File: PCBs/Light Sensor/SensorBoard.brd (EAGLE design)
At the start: 69.8 x 56.8 mm, 21 parts, among them J1 AVR_SPI_PRG_6PTH

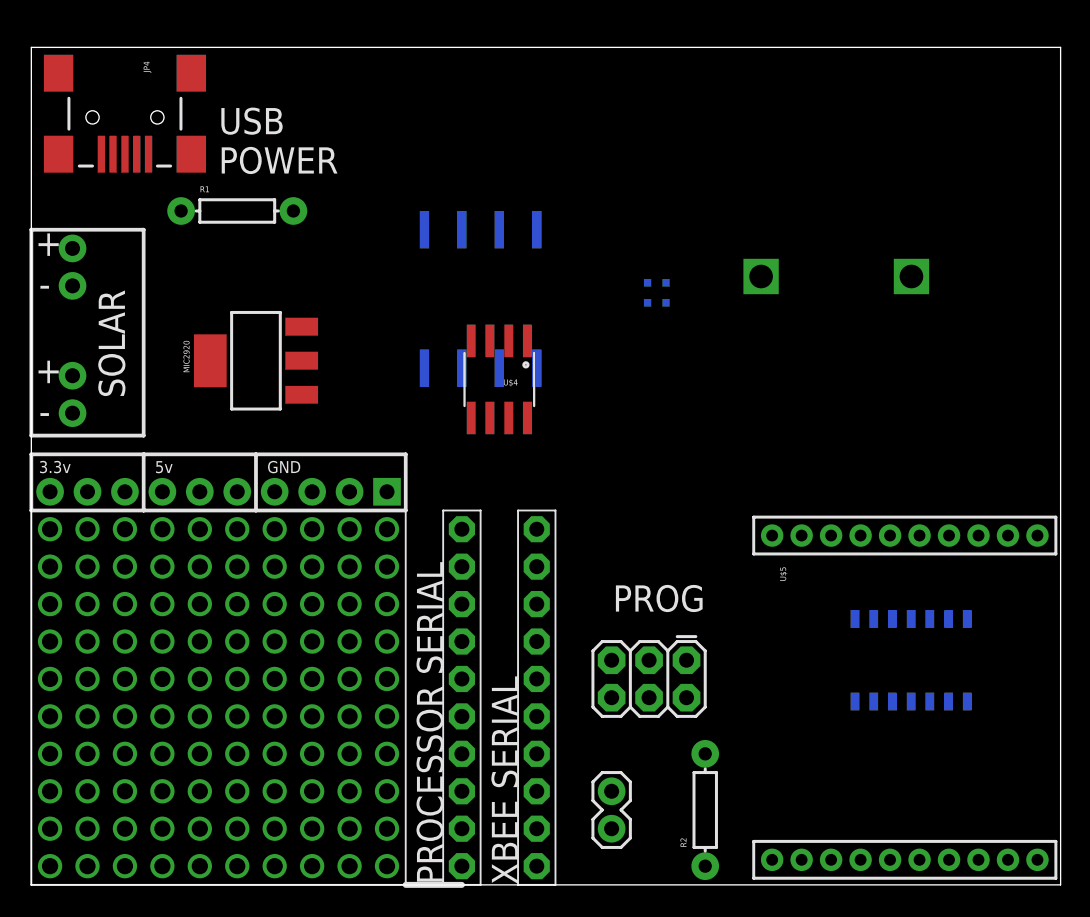
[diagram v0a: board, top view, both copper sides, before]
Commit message: Working layout
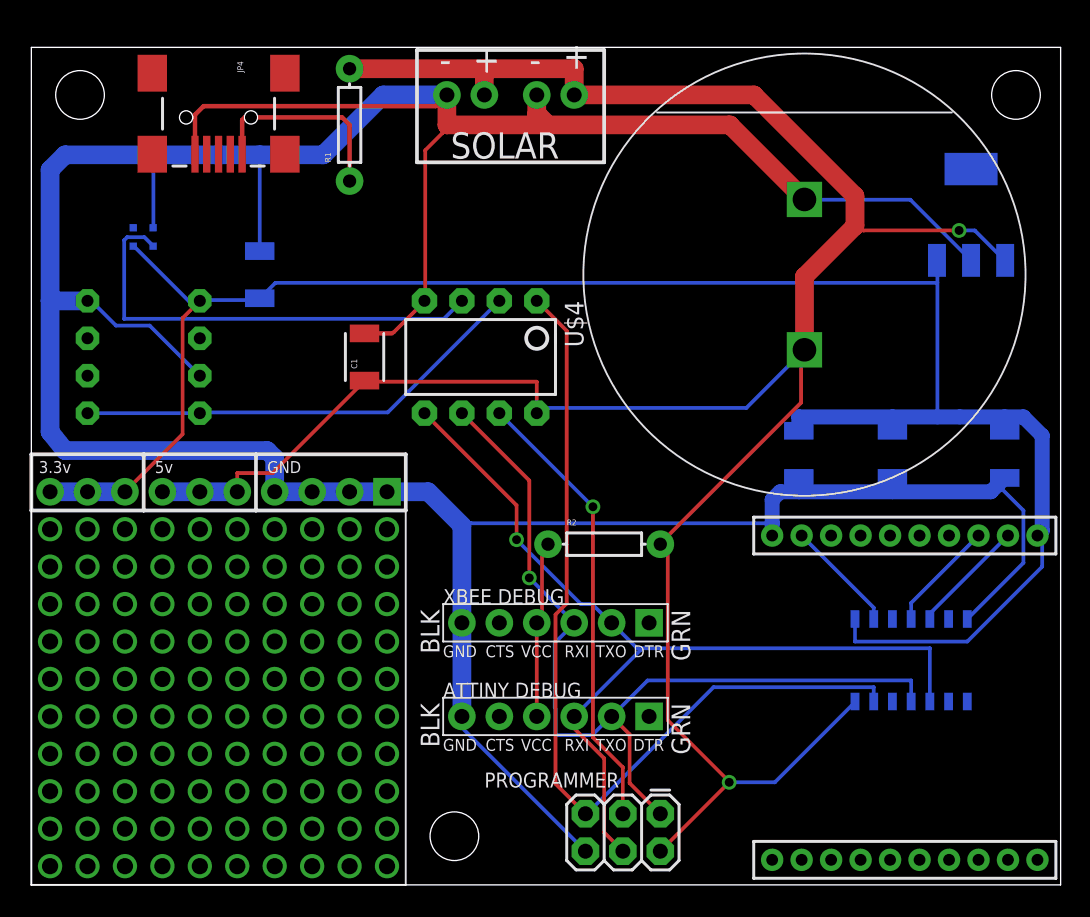
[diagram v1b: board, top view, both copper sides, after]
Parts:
- removed JP1: M02PTH, SparkFun-Connectors:1X02
- removed U$2, U$6: PINHD-1X10, adafruit:1X10-BIG
- added C1, C2, C3, C4, C5: (no value), SparkFun-Capacitors:1210
- added STANDOFF1, STANDOFF2, STANDOFF3: STAND-OFF, SparkFun-Electromechanical:STAND-OFF
- added TINY, XBEE: FTDI_DEVICE, SparkFun-Connectors:FTDI_DEVICE_SIDE
- U$1: value OPT101SMD -> OPT101TH; device MyLibrary:PDSO-U8 -> MyLibrary:DIL08
- U$4: value ATTINY85SMD -> TINY85-20-DIP; device MyLibrary:SO08 -> SparkFun-DigitalIC:DIP08
- moved MIC2920 49.5 mm to (63.8, 45.5), flipped to the bottom, turned to 0 degrees
- moved JP2 35.6 mm to (36.8, 53.6), turned to 180 degrees
- moved U$3 35.2 mm to (8.38, 44.7), turned to 270 degrees
- moved JP3 33.8 mm to (30.7, 53.6), turned to 180 degrees
- moved U$1 20.9 mm to (7.62, 35.8), turned to 270 degrees
- moved R2 19.3 mm to (38.9, 23.1), turned to 0 degrees
- moved J1 10.6 mm to (42.7, 4.83)
- moved R1 9.60 mm to (21.6, 51.6), turned to 90 degrees
- moved JP4 6.35 mm to (12.7, 52.1)
- moved U$7 2.16 mm to (52.5, 41.4), flipped to the top, turned to 90 degrees
- moved U$4 1.98 mm to (30.5, 35.8)
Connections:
- removed net MISO/TINY_TX: J1.1, U$4.6, U1.11
- removed net MOSI/TINY_RX: J1.4, U$4.5, U1.10
- removed net N$3: U$2.4, U$6.3
- removed net N$4: R2.P$1, U$2.1, U$2.10, U$2.5, U$6.1, U$6.10, U$6.5
- removed net N$5: JP1.2, U1.8
- removed net RESET: J1.5, U$4.1, U1.12
- removed net TINY_DTR: U$4.3, U1.13
- removed net XBEE_RESET: U$5.5, U1.3
- new net MISO/TINY_RX: J1.1, TINY.P$2, U$4.6, U1.11, XBEE.P$3
- new net MOSI/TINY_TX: J1.4, TINY.P$3, U$4.5, U1.10, XBEE.P$2
- new net RST/TINY_DTR: J1.5, U$4.1, U1.13
- net 3.3V: now also C2.1, C3.1, C4.1, C5.1
- net 5V: now also C1.1
- net APDS_9008: now also U$4.3; no longer U$4.2
- net GND: now also C1.2, C2.2, C3.2, C4.2, C5.2, TINY.P$6, XBEE.P$6; no longer JP1.1, U$2.7, U$6.7
- net N$2: now also R2.P$1, TINY.P$4, XBEE.P$4; no longer U$2.3, U$6.4
- net OPT_101: now also U$4.2; no longer U$4.7
- net SCK: now also U$4.7
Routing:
- net GND: track 0.00 -> 262.9 mm
- net 5V: track 0.00 -> 169.3 mm, vias 0 -> 2
- net 3.3V: track 0.00 -> 133.4 mm
- net MOSI/TINY_TX: track 0.00 -> 62.9 mm, vias 0 -> 1
- net RST/TINY_DTR: track 0.00 -> 60.9 mm
- net MISO/TINY_RX: track 0.00 -> 60.6 mm, vias 0 -> 1
- net OPT_101: track 0.00 -> 31.1 mm
- net APDS_9008: track 0.00 -> 31.1 mm
- net SCK: track 0.00 -> 30.6 mm, vias 0 -> 1
- net N$1: track 0.00 -> 13.7 mm
- net N$2: track 0.00 -> 12.0 mm
- net XBEE_TX: track 0.00 -> 7.86 mm
- net XBEE_DTR: track 0.00 -> 7.69 mm
- net XBEE_RX: track 0.00 -> 7.55 mm
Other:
- board text added: "ATTINY DEBUG"
- board text added: "PROGRAMMER"
- board text added: "XBEE DEBUG"
- board text removed: "PROCESSOR SERIAL"
- board text removed: "PROG"
- board text removed: "USB POWER"
- board text removed: "XBEE SERIAL"
